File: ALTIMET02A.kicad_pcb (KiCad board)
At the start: 2 copper layers, 40.1 x 30.5 mm, 15 parts, among them IC1 MS561101BA03-50, J1 HEADER_2x03_PARALLEL, J2 HEADER_2x03, J3 HEADER_2x05_PARALLEL

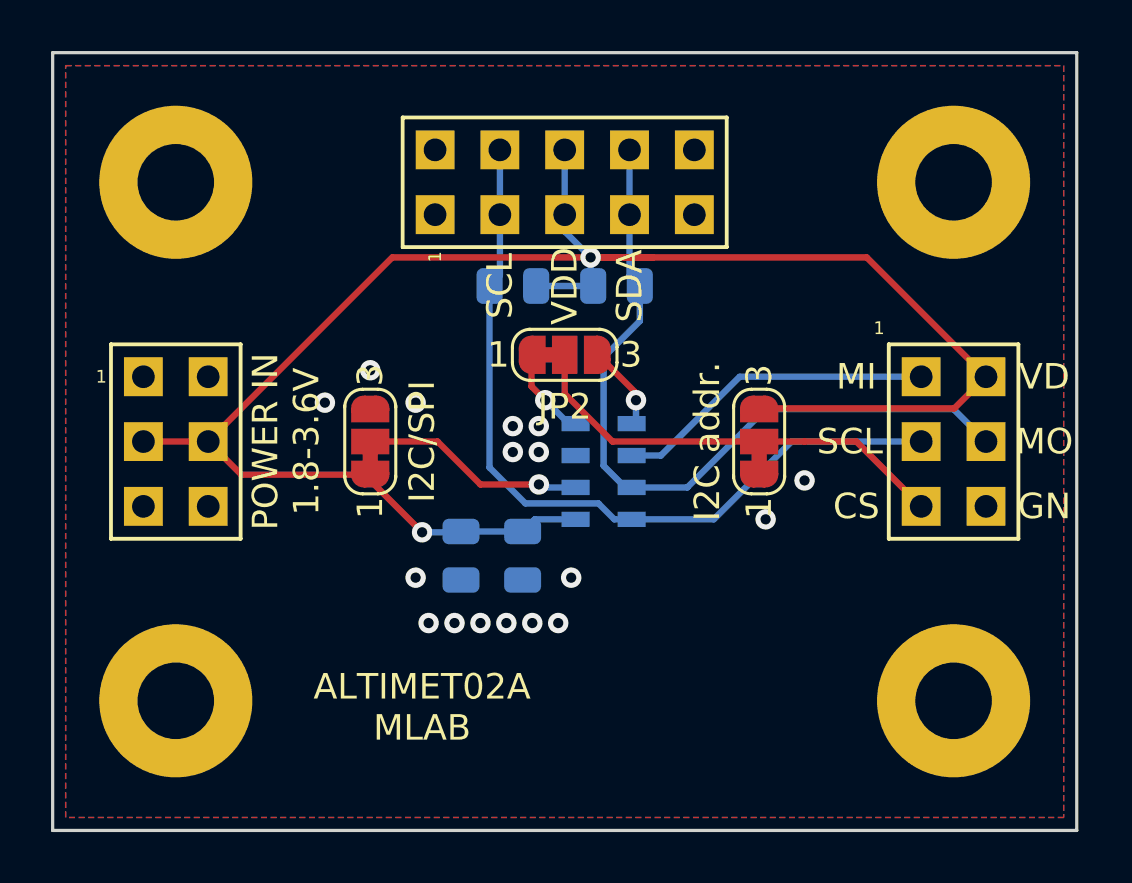
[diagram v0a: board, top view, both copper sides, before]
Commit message: 3x1 layout
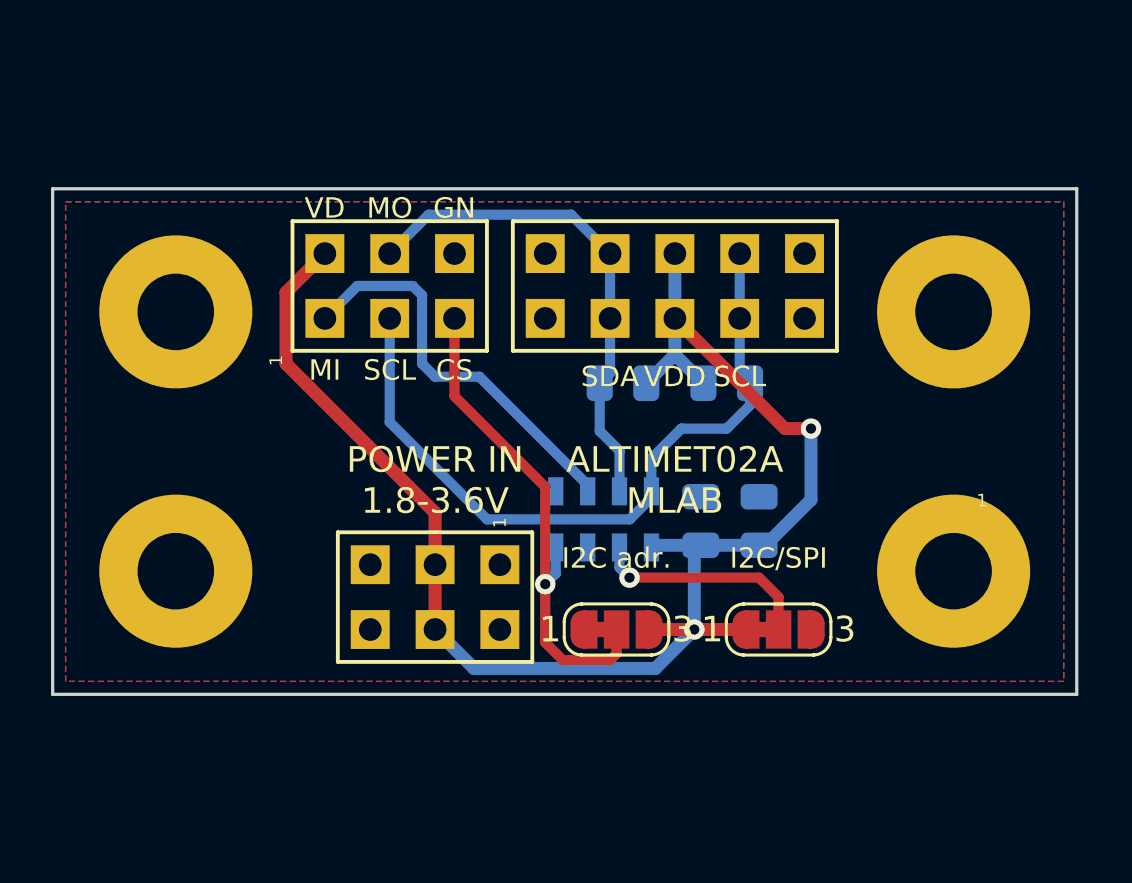
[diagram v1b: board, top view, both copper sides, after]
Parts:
- removed JP2: SolderJumper_3_Bridged123, Jumper:SolderJumper-3_P1.3mm_Bridged12_RoundedPad1.0x1.5mm_NumberLabels
- R1, R2: value 10k -> DNF
- moved J2 22.9 mm to (125.2, 100.6), turned to 90 degrees
- moved JP1 17.6 mm to (140.5, 114.0), turned to 0 degrees
- moved J1 11.8 mm to (127.0, 112.8), turned to -90 degrees
- moved C1 9.50 mm to (137.4, 109.8), turned to 90 degrees
- moved C2 9.37 mm to (139.7, 109.8), turned to 90 degrees
- moved JP3 9.25 mm to (134.1, 114.0), turned to 0 degrees
- moved R1 9.21 mm to (138.4, 104.4), turned to 0 degrees
- moved J3 5.93 mm to (136.4, 100.6), turned to -90 degrees
- moved H1 5.08 mm to (147.3, 111.8)
- moved H2 5.08 mm to (116.8, 111.8)
- moved H3 5.08 mm to (147.3, 101.6)
- moved H4 5.08 mm to (116.8, 101.6)
- moved R2 3.82 mm to (134.4, 104.4), turned to 180 degrees
- moved IC1 1.88 mm to (133.6, 109.7), turned to 90 degrees
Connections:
- IC1 pad 4: Net-(IC1-Pad4) -> CS/A
- IC1 pad 5: Net-(IC1-Pad5) -> unconnected-(IC1-Pad5)
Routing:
- net VDD: track 74.4 -> 60.4 mm
- net MOSI/SDA: track 30.3 -> 19.7 mm
- net Net-(IC1-Pad5): track 3.71 -> 0.00 mm, vias 1 -> 0
- net Net-(IC1-Pad4): track 3.57 -> 0.00 mm, vias 1 -> 0
- net MISO: track 12.6 -> 16.1 mm
- net SCLK: track 31.9 -> 28.6 mm
- net CS/A: track 17.3 -> 19.9 mm, vias 0 -> 1
- net GND: vias 17 -> 0
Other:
- board size 40.1 x 30.5 mm -> 40.1 x 19.8 mm
- board text added: "I2C adr."
- board text removed: "I2C addr."
